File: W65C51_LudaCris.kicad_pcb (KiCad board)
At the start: 2 copper layers, 167.6 x 111.2 mm, 21 parts, among them J1 USB_RST, J2 USB_C, J3 BB816_BreakoutA27_PCIex16, J3 I2C, J5 USB_Status, J6 I2C, J7 I2C, U1 W65C51NxP, U10 74HC191, U11 ATF22V10, U12 ATF22V10, U13 74HC138, U14 74HC283, U17 MCP2221AxP, U18 MAX232, U19 74HC191, U4 74HC191, U5 74HC191, U6 1.8432 MHz, U8 74HC573, U9 74HC191

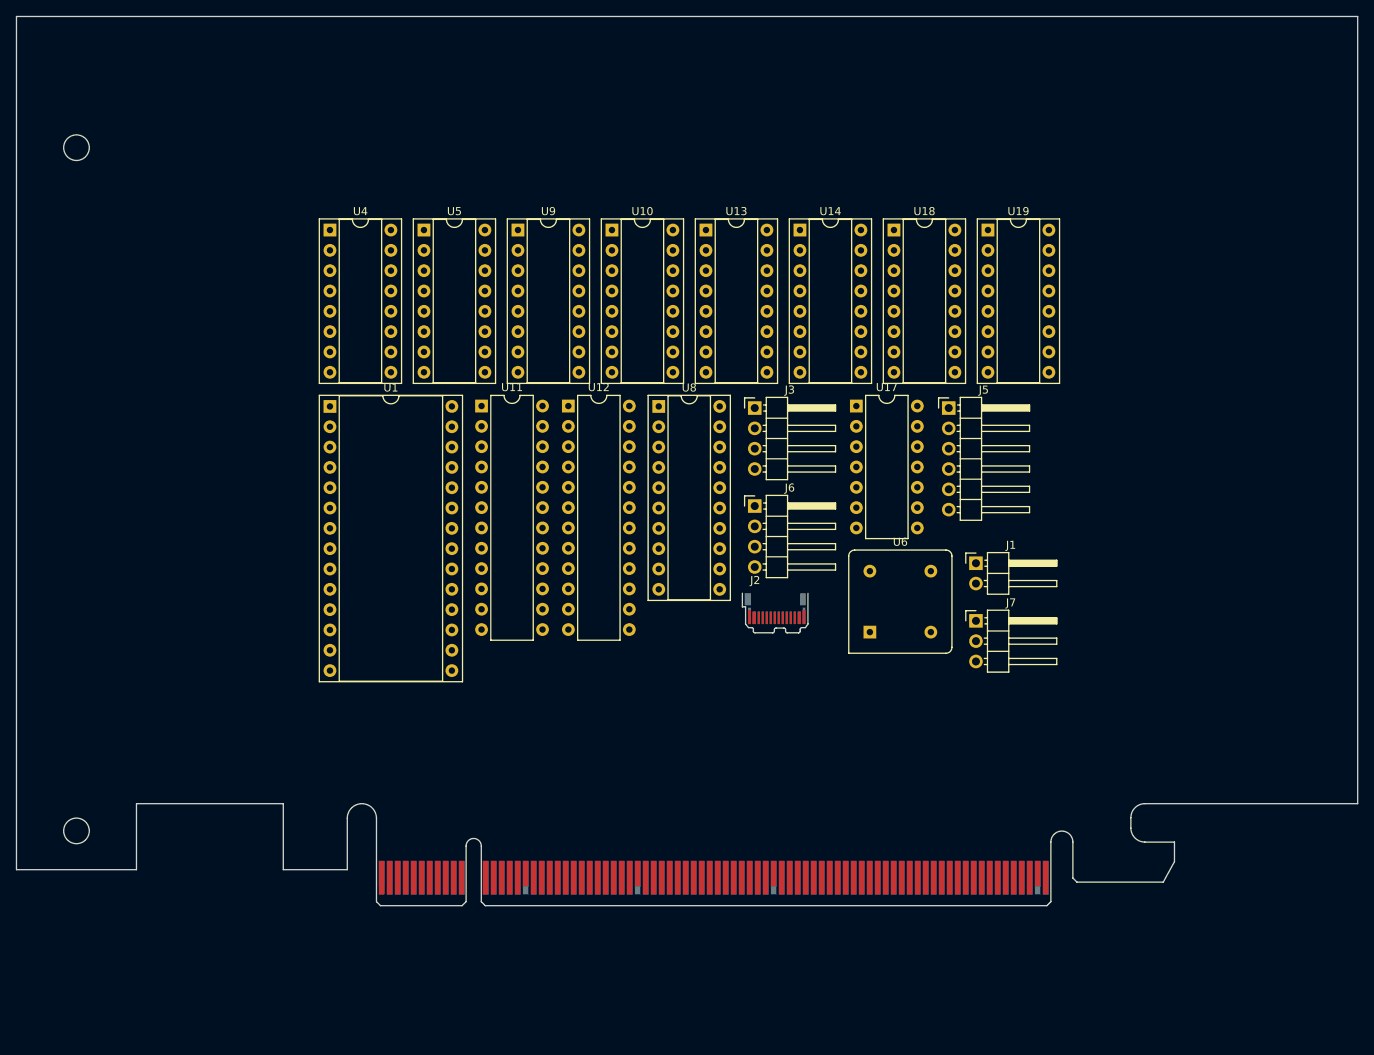
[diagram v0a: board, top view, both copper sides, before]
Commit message: GAL PLD
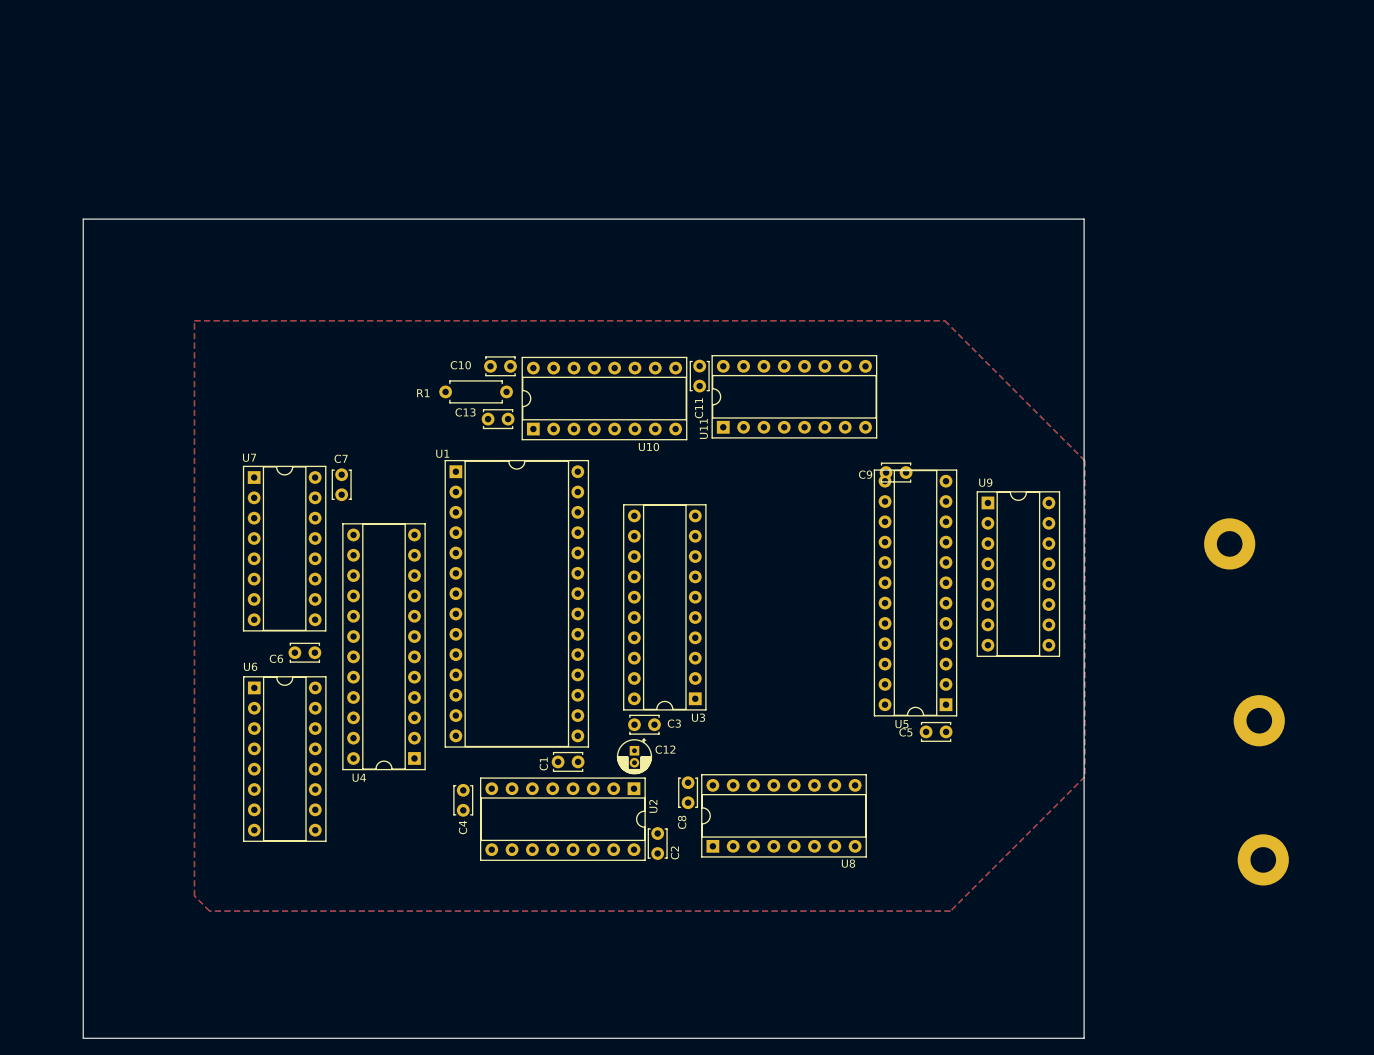
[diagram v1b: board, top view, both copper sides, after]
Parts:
- removed J1: USB_RST, Connector_PinHeader_2.54mm:PinHeader_1x02_P2.54mm_Horizontal
- removed J2: USB_C, Connector_USB:USB_C_Plug_JAE_DX07P024AJ1
- removed J3, J6: I2C, Connector_PinHeader_2.54mm:PinHeader_1x04_P2.54mm_Horizontal
- removed J3: BB816_BreakoutA27_PCIex16, BB816-MATX-PCIE:PCIexpress_x16_HW_FH
- removed J5: USB_Status, Connector_PinHeader_2.54mm:PinHeader_1x06_P2.54mm_Horizontal
- removed J7: I2C, Connector_PinHeader_2.54mm:PinHeader_1x03_P2.54mm_Horizontal
- removed U12: ATF22V10, Package_DIP:DIP-24_W7.62mm
- removed U13: 74HC138, Package_DIP:DIP-16_W7.62mm_Socket
- removed U14: 74HC283, Package_DIP:DIP-16_W7.62mm_Socket
- removed U17: MCP2221AxP, Package_DIP:DIP-14_W7.62mm
- removed U18: MAX232, Package_DIP:DIP-16_W7.62mm_Socket
- removed U19: 74HC191, Package_DIP:DIP-16_W7.62mm_Socket
- added C1: 100nF, Capacitor_THT:C_Disc_D3.4mm_W2.1mm_P2.50mm, F.Cu at (127.8, 132.8)
- added C10: 100nF, Capacitor_THT:C_Disc_D3.4mm_W2.1mm_P2.50mm, F.Cu at (119.3, 83.3)
- added C11: 100nF, Capacitor_THT:C_Disc_D3.4mm_W2.1mm_P2.50mm, F.Cu at (142.9, 83.3)
- added C12: 10uF, Capacitor_THT:CP_Radial_D4.0mm_P1.50mm, F.Cu at (134.8, 131.4)
- added C13: 1nF, Capacitor_THT:C_Disc_D3.4mm_W2.1mm_P2.50mm, F.Cu at (119.0, 89.9)
- added C2: 100nF, Capacitor_THT:C_Disc_D3.4mm_W2.1mm_P2.50mm, F.Cu at (137.7, 144.2)
- added C3: 100nF, Capacitor_THT:C_Disc_D3.4mm_W2.1mm_P2.50mm, F.Cu at (134.8, 128.1)
- added C4: 100nF, Capacitor_THT:C_Disc_D3.4mm_W2.1mm_P2.50mm, F.Cu at (113.4, 136.3)
- added C5: 100nF, Capacitor_THT:C_Disc_D3.4mm_W2.1mm_P2.50mm, F.Cu at (173.8, 129.0)
- added C6: 100nF, Capacitor_THT:C_Disc_D3.4mm_W2.1mm_P2.50mm, F.Cu at (94.8, 119.1)
- added C7: 100nF, Capacitor_THT:C_Disc_D3.4mm_W2.1mm_P2.50mm, F.Cu at (98.2, 96.8)
- added C8: 100nF, Capacitor_THT:C_Disc_D3.4mm_W2.1mm_P2.50mm, F.Cu at (141.5, 135.3)
- added C9: 100nF, Capacitor_THT:C_Disc_D3.4mm_W2.1mm_P2.50mm, F.Cu at (168.8, 96.6)
- added H1: MountingHole_Pad, MountingHole:MountingHole_3.2mm_M3_Pad, F.Cu at (209.2, 105.5)
- added H2: MountingHole_Pad, MountingHole:MountingHole_3.2mm_M3_Pad, F.Cu at (213.4, 145.0)
- added H3: MountingHole_Pad, MountingHole:MountingHole_3.2mm_M3_Pad, F.Cu at (212.9, 127.6)
- added R1: 50, Resistor_THT:R_Axial_DIN0207_L6.3mm_D2.5mm_P7.62mm_Horizontal, F.Cu at (118.8, 86.5)
- added U2: 74HC138, Package_DIP:DIP-16_W7.62mm_Socket, F.Cu at (134.7, 136.1)
- added U3: 74HC573, Package_DIP:DIP-20_W7.62mm_Socket, F.Cu at (142.4, 124.9)
- added U7: 74HC191, Package_DIP:DIP-16_W7.62mm_Socket, F.Cu at (87.3, 97.2)
- U10: value 74HC191 -> 74HC283
- U11: value ATF22V10 -> 74HC191; footprint Package_DIP:DIP-24_W7.62mm -> Package_DIP:DIP-16_W7.62mm_Socket
- U4, U5: value 74HC191 -> ATF22V10; footprint Package_DIP:DIP-16_W7.62mm_Socket -> Package_DIP:DIP-24_W7.62mm_Socket
- U6: value 1.8432 MHz -> 74HC191; footprint Oscillator:Oscillator_DIP-8 -> Package_DIP:DIP-16_W7.62mm_Socket
- U8: value 74HC573 -> 74HC191; footprint Package_DIP:DIP-20_W7.62mm_Socket -> Package_DIP:DIP-16_W7.62mm_Socket
- moved U5 88.2 mm to (173.7, 125.6), turned to 180 degrees
- moved U6 77.3 mm to (87.3, 123.5)
- moved U9 67.9 mm to (179.0, 100.4)
- moved U4 66.9 mm to (107.3, 132.3), turned to 180 degrees
- moved U8 55.4 mm to (144.6, 143.3), turned to 90 degrees
- moved U11 30.3 mm to (145.9, 90.9), turned to 90 degrees
- moved U10 26.7 mm to (122.2, 91.1), turned to 90 degrees
- moved U1 17.7 mm to (112.5, 96.5)
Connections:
- net /~{IRQ1} renamed /~{IRQ}
- U1 pad 10: TxD -> /TxD
- U1 pad 11: unconnected-(U1-~{DTR}-Pad11) -> /~{DTR}
- U1 pad 12: RxD -> /RxD
- U1 pad 13: /A0 -> /RS0
- U1 pad 14: /A1 -> /RS1
- U1 pad 16: GND -> /~{DCD}
- U1 pad 2: VCC -> /CS1
- U1 pad 28: /~{WR} -> /R~{W}
- U1 pad 3: /~{IOCS1} -> /~{CS2}
- U1 pad 5: unconnected-(U1-RxC-Pad5) -> /RxC
- U1 pad 7: unconnected-(U1-XTAL2-Pad7) -> /XTAL2
- U1 pad 8: unconnected-(U1-~{RTS}-Pad8) -> /~{RTS}
- U1 pad 9: GND -> /~{CTS}
- U10 pad 1: /Q9 -> Net-(U10-S2)
- U10 pad 10: /Q10 -> Net-(U10-S4)
- U10 pad 11: /~{BAUD_LOAD} -> GND
- U10 pad 12: unconnected-(U10-MAX/MIN-Pad12) -> GND
- U10 pad 13: Net-(U10-~{RCO}) -> Net-(U10-S3)
- U10 pad 14: Net-(U10-CLK) -> GND
- U10 pad 15: /Q8 -> VCC
- U10 pad 2: unconnected-(U10-Qb-Pad2) -> VCC
- U10 pad 3: unconnected-(U10-Qa-Pad3) -> /CR6
- U10 pad 4: /~{CTEN} -> Net-(U10-S1)
- U10 pad 5: VCC -> /CR5
- U10 pad 6: unconnected-(U10-Qc-Pad6) -> GND
- U10 pad 7: unconnected-(U10-Qd-Pad7) -> /CR7
- U10 pad 9: /Q11 -> unconnected-(U10-C4-Pad9)
- U11 pad 1: VCC -> Net-(U10-S2)
- U11 pad 10: GND -> Net-(U10-S3)
- U11 pad 11: GND -> /~{TX_START}
- U11 pad 12: GND -> unconnected-(U11-MAX/MIN-Pad12)
- U11 pad 13: GND -> /~{TX_COMPLETE}
- U11 pad 14: /~{CTEN} -> /~{BAUD_CLK}
- U11 pad 15: /CTL_REG_WR -> Net-(U10-S1)
- U11 pad 16: /Q8 -> VCC
- U11 pad 2: /CR0 -> unconnected-(U11-Qb-Pad2)
- U11 pad 3: /CR1 -> unconnected-(U11-Qa-Pad3)
- U11 pad 4: /CR2 -> /~{CTEN}
- U11 pad 5: /CR3 -> VCC
- U11 pad 9: GND -> Net-(U10-S4)
- U4 pad 1: Net-(U14-S2) -> VCC
- U4 pad 10: Net-(U14-S3) -> GND
- U4 pad 11: /~{TX_START} -> GND
- U4 pad 12: unconnected-(U4-MAX/MIN-Pad12) -> GND
- U4 pad 13: /~{TX_COMPLETE} -> /~{BAUD_CLK}
- U4 pad 14: /~{BAUD_CLK} -> /~{DSR}
- U4 pad 15: Net-(U14-S1) -> /~{BAUD_LOAD}
- U4 pad 16: VCC -> /~{CTEN}
- U4 pad 2: unconnected-(U4-Qb-Pad2) -> /CR0
- U4 pad 3: unconnected-(U4-Qa-Pad3) -> /CR1
- U4 pad 4: /~{CTEN} -> /CR2
- U4 pad 5: VCC -> /CR3
- U4 pad 6: unconnected-(U4-Qc-Pad6) -> /~{CTL_REG_WR}
- U4 pad 7: unconnected-(U4-Qd-Pad7) -> /~{TX_START}
- U4 pad 8: GND -> /~{TX_COMPLETE}
- U4 pad 9: Net-(U14-S4) -> GND
- U5 pad 1: /Q5 -> VCC
- U5 pad 10: /Q6 -> GND
- U5 pad 11: /~{BAUD_LOAD} -> GND
- U5 pad 12: unconnected-(U5-MAX/MIN-Pad12) -> GND
- U5 pad 13: Net-(U10-CLK) -> GND
- U5 pad 14: Net-(U19-~{RCO}) -> unconnected-(U5-I/O-Pad14)
- U5 pad 15: /Q4 -> unconnected-(U5-I/O-Pad15)
- U5 pad 16: unconnected-(U5-VCC-Pad16) -> /Q8
- U5 pad 2: unconnected-(U5-Qb-Pad2) -> /CR0
- U5 pad 3: unconnected-(U5-Qa-Pad3) -> /CR1
- U5 pad 4: /~{CTEN} -> /CR2
- U5 pad 5: VCC -> /CR3
- U5 pad 6: unconnected-(U5-Qc-Pad6) -> GND
- U5 pad 7: unconnected-(U5-Qd-Pad7) -> GND
- U5 pad 9: /Q7 -> GND
- U6 pad 1: VCC -> GND
- U6 pad 4: GND -> /~{CTEN}
- U6 pad 5: /XTAL1 -> VCC
- U6 pad 8: VCC -> GND
- U8 pad 1: GND -> /Q9
- U8 pad 10: GND -> /Q10
- U8 pad 11: /CTL_REG_WR -> /~{BAUD_LOAD}
- U8 pad 12: /CR7 -> unconnected-(U8-MAX/MIN-Pad12)
- U8 pad 13: /CR6 -> Net-(U8-~{RCO})
- U8 pad 14: /CR5 -> Net-(U7-~{RCO})
- U8 pad 15: /CR4 -> /Q8
- U8 pad 16: /CR3 -> VCC
- U8 pad 2: /D0 -> unconnected-(U8-Qb-Pad2)
- U8 pad 3: /D1 -> unconnected-(U8-Qa-Pad3)
- U8 pad 4: /D2 -> /~{CTEN}
- U8 pad 5: /D3 -> VCC
- U8 pad 6: /D4 -> unconnected-(U8-Qc-Pad6)
- U8 pad 7: /D5 -> unconnected-(U8-Qd-Pad7)
- U8 pad 8: /D6 -> GND
- U8 pad 9: /D7 -> /Q11
- U9 pad 14: Net-(U10-~{RCO}) -> Net-(U8-~{RCO})
- U9 pad 16: unconnected-(U9-VCC-Pad16) -> VCC
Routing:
- added copper zone on In1.Cu, net GND
- added copper zone on In2.Cu, net GND
- added copper zone on B.Cu, net VCC
- added copper zone on F.Cu, net VCC
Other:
- board size 167.6 x 111.2 mm -> 125.1 x 102.4 mm
- copper layers 2 -> 4
